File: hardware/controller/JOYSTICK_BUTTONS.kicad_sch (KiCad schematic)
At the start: 18 parts, among them SW101 UP, SW102 LEFT, SW103 DOWN, SW104 RIGHT

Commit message: done but need to add stitching vias
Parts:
- TP106, TP107, TP108, TP109: footprint TestPoint:TestPoint_Pad_1.0x1.0mm -> SamacSys_Parts:TestPoint_Pad_1.0x1.0mm
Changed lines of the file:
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@@
 			)
 		)
-		(property "Footprint" "TestPoint:TestPoint_Pad_1.0x1.0mm"
+		(property "Footprint" "SamacSys_Parts:TestPoint_Pad_1.0x1.0mm"
 			(at 134.62 55.88 0)
 			(effects
@@
 			)
 		)
-		(property "Footprint" "TestPoint:TestPoint_Pad_1.0x1.0mm"
+		(property "Footprint" "SamacSys_Parts:TestPoint_Pad_1.0x1.0mm"
 			(at 134.62 93.98 0)
 			(effects
@@
 			)
 		)
-		(property "Footprint" "TestPoint:TestPoint_Pad_1.0x1.0mm"
+		(property "Footprint" "SamacSys_Parts:TestPoint_Pad_1.0x1.0mm"
 			(at 134.62 105.41 0)
 			(effects
@@
 			)
 		)
-		(property "Footprint" "TestPoint:TestPoint_Pad_1.0x1.0mm"
+		(property "Footprint" "SamacSys_Parts:TestPoint_Pad_1.0x1.0mm"
 			(at 134.62 44.45 0)
 			(effects

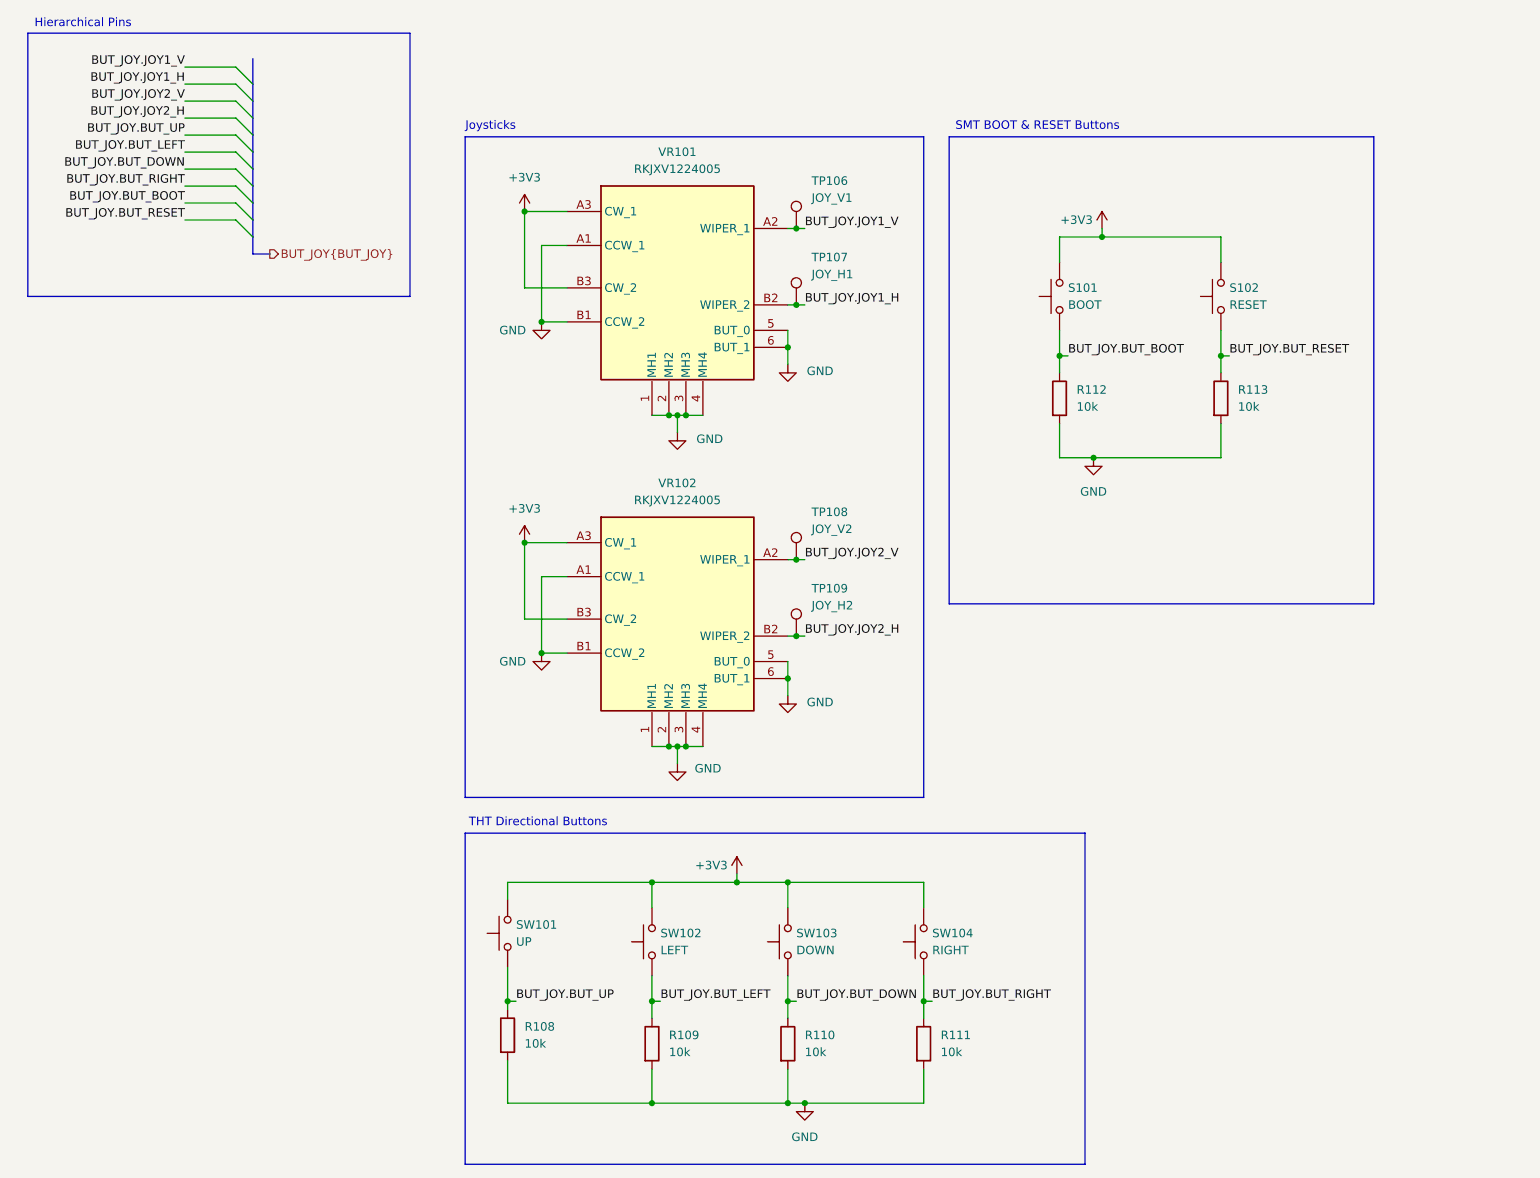
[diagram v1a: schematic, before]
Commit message: forgor
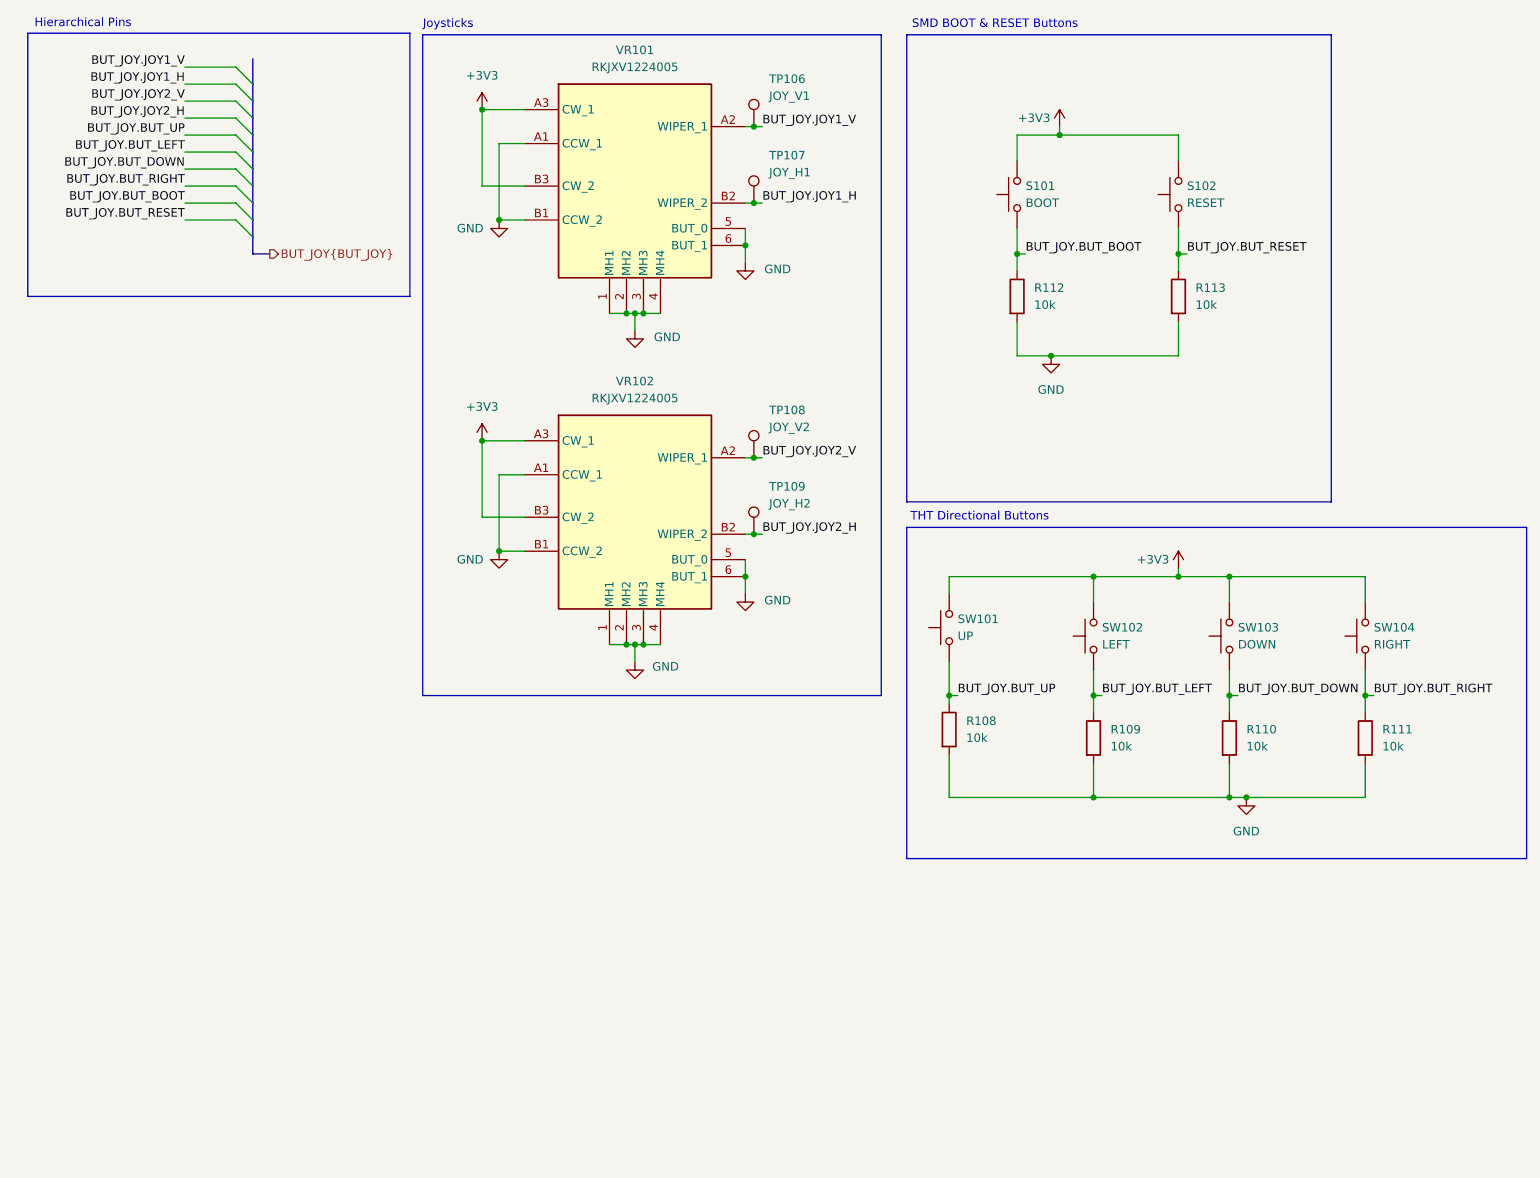
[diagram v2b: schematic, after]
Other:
- note added: "SMD BOOT & RESET Buttons"
- note removed: "SMT BOOT & RESET Buttons"
- moved on the sheet: R108, R109, R110, R111, R112, R113, S101, S102, SW101, SW102, SW103, SW104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
